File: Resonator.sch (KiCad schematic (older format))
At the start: 29 parts, among them J1 Conn_01x04_Male, SW1 Rotary_Encoder_Switch, SW2 SW_Push, U1 STM32H750VBTx, U2 AT25xxx, U3 IPS240x240, Y1 ABM8G-25.000MHZ-18-D2Y-T

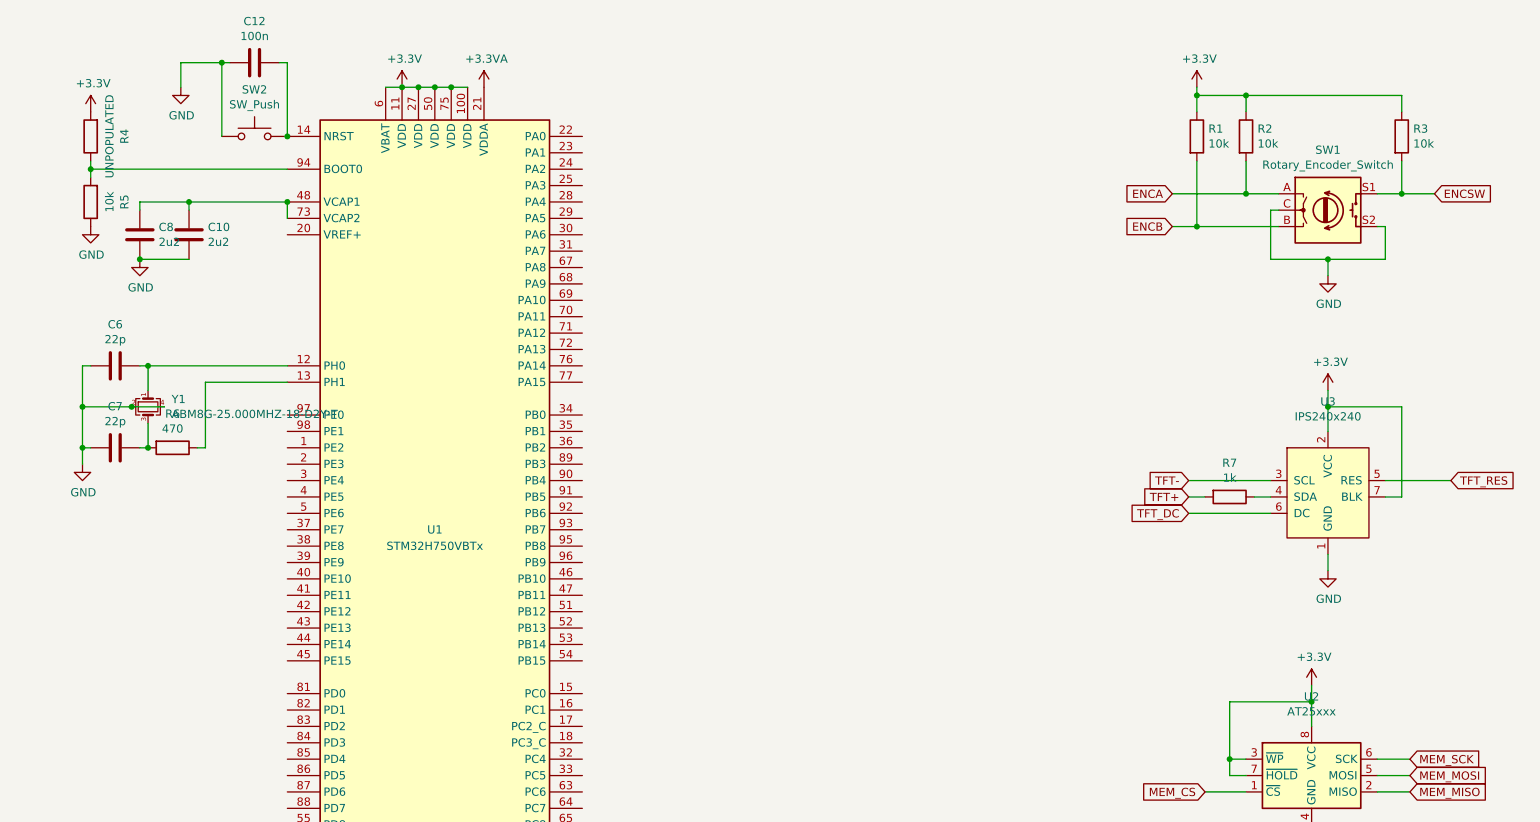
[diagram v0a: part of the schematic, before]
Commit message: Re-annotation.
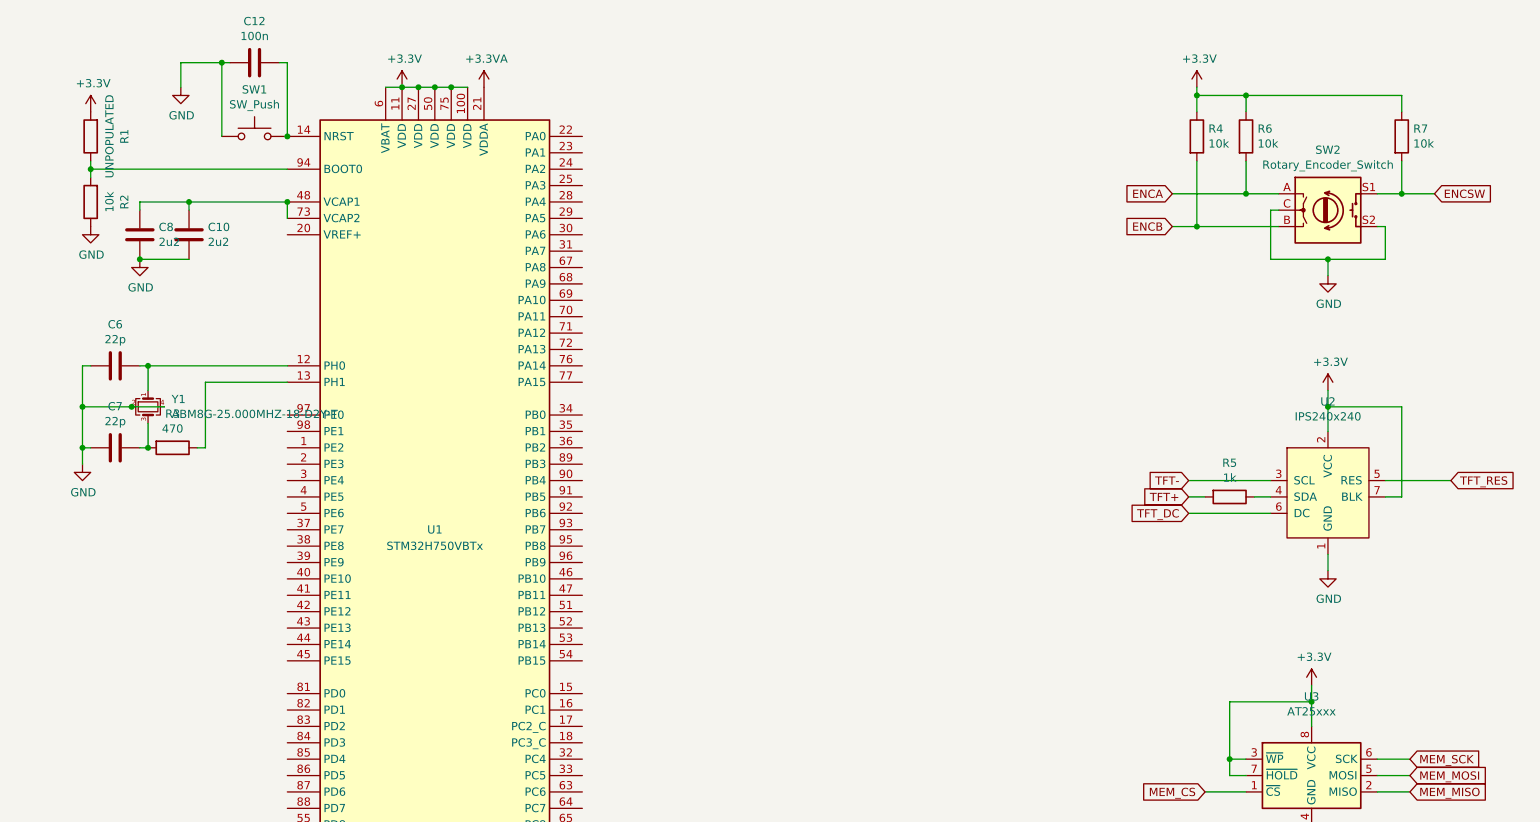
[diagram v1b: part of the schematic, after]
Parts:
- renumbered R4 to R1, R5 to R2, R6 to R3, R1 to R4, R7 to R5, R2 to R6, R3 to R7, SW2 to SW1, SW1 to SW2, U3 to U2, U2 to U3
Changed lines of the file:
@@
 $Descr A3 16535 11693
 encoding utf-8
-Sheet 1 6
+Sheet 1 11
 Title "Resonator"
 Date "2021-11-21"
@@
 Connection ~ 7650 2750
 $Comp
-L power:+3.3V #PWR013
+L power:+3.3V #PWR012
 U 1 1 61D958D9
 P 7650 2750
-F 0 "#PWR013" H 7650 2600 50  0001 C CNN
+F 0 "#PWR012" H 7650 2600 50  0001 C CNN
 F 1 "+3.3V" H 7665 2923 50  0000 C CNN
 F 2 "" H 7650 2750 50  0001 C CNN
@@
 $EndComp
 $Comp
-L power:+3.3VA #PWR016
+L power:+3.3VA #PWR015
 U 1 1 61D96DEA
 P 8150 2750
-F 0 "#PWR016" H 8150 2600 50  0001 C CNN
+F 0 "#PWR015" H 8150 2600 50  0001 C CNN
 F 1 "+3.3VA" H 8165 2923 50  0000 C CNN
 F 2 "" H 8150 2750 50  0001 C CNN
@@
 $EndComp
 $Comp
-L power:GND #PWR012
+L power:GND #PWR011
 U 1 1 61D9B5CB
 P 7550 8250
-F 0 "#PWR012" H 7550 8000 50  0001 C CNN
+F 0 "#PWR011" H 7550 8000 50  0001 C CNN
 F 1 "GND" H 7555 8077 50  0000 C CNN
 F 2 "" H 7550 8250 50  0001 C CNN
@@
 	6950 3550 6950 3450
 $Comp
-L power:GND #PWR010
+L power:GND #PWR09
 U 1 1 61DA19D2
 P 6050 3800
-F 0 "#PWR010" H 6050 3550 50  0001 C CNN
+F 0 "#PWR09" H 6050 3550 50  0001 C CNN
 F 1 "GND" H 6055 3627 50  0000 C CNN
 F 2 "" H 6050 3800 50  0001 C CNN
@@
 Connection ~ 6050 3800
 $Comp
-L power:+3V3 #PWR04
+L power:+3V3 #PWR03
 U 1 1 61DAD533
 P 4050 10300
-F 0 "#PWR04" H 4050 10150 50  0001 C CNN
+F 0 "#PWR03" H 4050 10150 50  0001 C CNN
 F 1 "+3V3" H 4065 10473 50  0000 C CNN
 F 2 "" H 4050 10300 50  0001 C CNN
@@
 	4050 10300 4200 10300
 $Comp
-L power:GND #PWR05
+L power:GND #PWR04
 U 1 1 61DAD53E
 P 4050 10600
-F 0 "#PWR05" H 4050 10350 50  0001 C CNN
+F 0 "#PWR04" H 4050 10350 50  0001 C CNN
 F 1 "GND" H 4055 10427 50  0000 C CNN
 F 2 "" H 4050 10600 50  0001 C CNN
@@
 $EndComp
 $Comp
-L Device:R R4
+L Device:R R1
 U 1 1 61DB7AD0
 P 5750 3050
-F 0 "R4" V 5543 3050 50  0000 C CNN
+F 0 "R1" V 5543 3050 50  0000 C CNN
 F 1 "UNPOPULATED" V 5634 3050 50  0000 C CNN
 F 2 "Resistor_SMD:R_0603_1608Metric" V 5680 3050 50  0001 C CNN
@@
 $EndComp
 $Comp
-L Switch:SW_Push SW2
+L Switch:SW_Push SW1
 U 1 1 61DBD527
 P 6750 3050
-F 0 "SW2" H 6750 3335 50  0000 C CNN
+F 0 "SW1" H 6750 3335 50  0000 C CNN
 F 1 "SW_Push" H 6750 3244 50  0000 C CNN
 F 2 "Button_Switch_THT:SW_PUSH_6mm" H 6750 3250 50  0001 C CNN
@@
 	6950 2600 6900 2600
 $Comp
-L power:GND #PWR011
+L power:GND #PWR010
 U 1 1 61DC8FB1
 P 6300 2750
-F 0 "#PWR011" H 6300 2500 50  0001 C CNN
+F 0 "#PWR010" H 6300 2500 50  0001 C CNN
 F 1 "GND" H 6305 2577 50  0000 C CNN
 F 2 "" H 6300 2750 50  0001 C CNN
@@
 	5700 4700 5700 4450
 $Comp
-L power:GND #PWR07
+L power:GND #PWR06
 U 1 1 61E01E16
 P 5700 5050
-F 0 "#PWR07" H 5700 4800 50  0001 C CNN
+F 0 "#PWR06" H 5700 4800 50  0001 C CNN
 F 1 "GND" H 5705 4877 50  0000 C CNN
 F 2 "" H 5700 5050 50  0001 C CNN
@@
 	7750 10300 7900 10300
 $Comp
-L power:GND #PWR015
+L power:GND #PWR014
 U 1 1 61E8662A
 P 7750 10600
-F 0 "#PWR015" H 7750 10350 50  0001 C CNN
+F 0 "#PWR014" H 7750 10350 50  0001 C CNN
 F 1 "GND" H 7755 10427 50  0000 C CNN
 F 2 "" H 7750 10600 50  0001 C CNN
@@
 	7750 10600 7900 10600
 $Comp
-L power:+3.3VA #PWR014
+L power:+3.3VA #PWR013
 U 1 1 61E8B8BA
 P 7750 10300
-F 0 "#PWR014" H 7750 10150 50  0001 C CNN
+F 0 "#PWR013" H 7750 10150 50  0001 C CNN
 F 1 "+3.3VA" H 7765 10473 50  0000 C CNN
 F 2 "" H 7750 10300 50  0001 C CNN
@@
 	7900 10600 8300 10600
 $Comp
-L Device:R R5
+L Device:R R2
 U 1 1 61ADEFE2
 P 5750 3450
-F 0 "R5" V 5543 3450 50  0000 C CNN
+F 0 "R2" V 5543 3450 50  0000 C CNN
 F 1 "10k" V 5634 3450 50  0000 C CNN
 F 2 "Resistor_SMD:R_0603_1608Metric" V 5680 3450 50  0001 C CNN
@@
 	6100 4800 6100 4950
 $Comp
-L Device:R R6
+L Device:R R3
 U 1 1 61AE0744
 P 6250 4950
-F 0 "R6" V 6043 4950 50  0000 C CNN
+F 0 "R3" V 6043 4950 50  0000 C CNN
 F 1 "470" V 6134 4950 50  0000 C CNN
 F 2 "Resistor_SMD:R_0603_1608Metric" V 6180 4950 50  0001 C CNN
@@
 	5750 3250 5750 3200
 $Comp
-L power:GND #PWR09
+L power:GND #PWR08
 U 1 1 61AF8BC1
 P 5750 3600
-F 0 "#PWR09" H 5750 3350 50  0001 C CNN
+F 0 "#PWR08" H 5750 3350 50  0001 C CNN
 F 1 "GND" H 5755 3427 50  0000 C CNN
 F 2 "" H 5750 3600 50  0001 C CNN
@@
 $EndComp
 $Comp
-L power:+3.3V #PWR08
+L power:+3.3V #PWR07
 U 1 1 61AF9828
 P 5750 2900
-F 0 "#PWR08" H 5750 2750 50  0001 C CNN
+F 0 "#PWR07" H 5750 2750 50  0001 C CNN
 F 1 "+3.3V" H 5765 3073 50  0000 C CNN
 F 2 "" H 5750 2900 50  0001 C CNN
@@
 P 13200 6950
 AR Path="/5DD41DD6/61DD28C6" Ref="U?"  Part="1"
-AR Path="/61DD28C6" Ref="U2"  Part="1"
+AR Path="/61DD28C6" Ref="U3"  Part="1"
 AR Path="/61DB1EC2/61DD28C6" Ref="U?"  Part="1"
-F 0 "U2" H 13200 7431 50  0000 C CNN
+F 0 "U3" H 13200 7431 50  0000 C CNN
 F 1 "AT25xxx" H 13200 7340 50  0000 C CNN
 F 2 "Package_SO:TSSOP-8_4.4x3mm_P0.65mm" H 13200 6950 50  0001 C CNN
@@
 P 13200 7350
 AR Path="/5DD41DD6/61DD28CC" Ref="#PWR?"  Part="1"
-AR Path="/61DD28CC" Ref="#PWR024"  Part="1"
+AR Path="/61DD28CC" Ref="#PWR018"  Part="1"
 AR Path="/61DB1EC2/61DD28CC" Ref="#PWR?"  Part="1"
-F 0 "#PWR024" H 13200 7100 50  0001 C CNN
+F 0 "#PWR018" H 13200 7100 50  0001 C CNN
 F 1 "GND" H 13205 7177 50  0000 C CNN
 F 2 "" H 13200 7350 50  0001 C CNN
@@
 P 13200 6400
 AR Path="/5DD41DD6/61DD28D3" Ref="#PWR?"  Part="1"
-AR Path="/61DD28D3" Ref="#PWR023"  Part="1"
+AR Path="/61DD28D3" Ref="#PWR017"  Part="1"
 AR Path="/61DB1EC2/61DD28D3" Ref="#PWR?"  Part="1"
-F 0 "#PWR023" H 13200 6250 50  0001 C CNN
+F 0 "#PWR017" H 13200 6250 50  0001 C CNN
 F 1 "+3.3V" H 13215 6573 50  0000 C CNN
 F 2 "" H 13200 6400 50  0001 C CNN
@@
 P 13300 3500
 AR Path="/5DD41DD6/61DE3E76" Ref="SW?"  Part="1"
-AR Path="/61DE3E76" Ref="SW1"  Part="1"
+AR Path="/61DE3E76" Ref="SW2"  Part="1"
 AR Path="/61DB1EC2/61DE3E76" Ref="SW?"  Part="1"
-F 0 "SW1" H 13300 3867 50  0000 C CNN
+F 0 "SW2" H 13300 3867 50  0000 C CNN
 F 1 "Rotary_Encoder_Switch" H 13300 3776 50  0000 C CNN
 F 2 "Rotary_Encoder:RotaryEncoder_Alps_EC11E-Switch_Vertical_H20mm" H 13150 3660 50  0001 C CNN
@@
 P 13300 3900
 AR Path="/5DD41DD6/61DE3E7C" Ref="#PWR?"  Part="1"
-AR Path="/61DE3E7C" Ref="#PWR03"  Part="1"
+AR Path="/61DE3E7C" Ref="#PWR019"  Part="1"
 AR Path="/61DB1EC2/61DE3E7C" Ref="#PWR?"  Part="1"
-F 0 "#PWR03" H 13300 3650 50  0001 C CNN
+F 0 "#PWR019" H 13300 3650 50  0001 C CNN
 F 1 "GND" H 13305 3727 50  0000 C CNN
 F 2 "" H 13300 3900 50  0001 C CNN
@@
 P 13750 3050
 AR Path="/61DB1EC2/61DE3E90" Ref="R?"  Part="1"
-AR Path="/61DE3E90" Ref="R3"  Part="1"
-F 0 "R3" H 13820 3096 50  0000 L CNN
+AR Path="/61DE3E90" Ref="R7"  Part="1"
+F 0 "R7" H 13820 3096 50  0000 L CNN
 F 1 "10k" H 13820 3005 50  0000 L CNN
 F 2 "Resistor_SMD:R_0603_1608Metric" V 13680 3050 50  0001 C CNN
@@
 P 12800 3050
 AR Path="/61DB1EC2/61DE3E96" Ref="R?"  Part="1"
-AR Path="/61DE3E96" Ref="R2"  Part="1"
-F 0 "R2" H 12870 3096 50  0000 L CNN
+AR Path="/61DE3E96" Ref="R6"  Part="1"
+F 0 "R6" H 12870 3096 50  0000 L CNN
 F 1 "10k" H 12870 3005 50  0000 L CNN
 F 2 "Resistor_SMD:R_0603_1608Metric" V 12730 3050 50  0001 C CNN
@@
 P 12500 3050
 AR Path="/61DB1EC2/61DE3E9C" Ref="R?"  Part="1"
-AR Path="/61DE3E9C" Ref="R1"  Part="1"
-F 0 "R1" H 12570 3096 50  0000 L CNN
+AR Path="/61DE3E9C" Ref="R4"  Part="1"
+F 0 "R4" H 12570 3096 50  0000 L CNN
 F 1 "10k" H 12570 3005 50  0000 L CNN
 F 2 "Resistor_SMD:R_0603_1608Metric" V 12430 3050 50  0001 C CNN
@@
 P 12500 2750
 AR Path="/61DB1EC2/61DE3EAB" Ref="#PWR?"  Part="1"
-AR Path="/61DE3EAB" Ref="#PWR01"  Part="1"
-F 0 "#PWR01" H 12500 2600 50  0001 C CNN
+AR Path="/61DE3EAB" Ref="#PWR016"  Part="1"
+F 0 "#PWR016" H 12500 2600 50  0001 C CNN
 F 1 "+3.3V" H 12515 2923 50  0000 C CNN
 F 2 "" H 12500 2750 50  0001 C CNN
@@
 P 5550 9350
 AR Path="/5DD41DD6/61DED307" Ref="#PWR?"  Part="1"
-AR Path="/61DED307" Ref="#PWR06"  Part="1"
+AR Path="/61DED307" Ref="#PWR05"  Part="1"
 AR Path="/61DB1EC2/61DED307" Ref="#PWR?"  Part="1"
-F 0 "#PWR06" H 5550 9100 50  0001 C CNN
+F 0 "#PWR05" H 5550 9100 50  0001 C CNN
 F 1 "GND" H 5555 9177 50  0000 C CNN
 F 2 "" H 5550 9350 50  0001 C CNN
@@
 P 12700 5250
 AR Path="/5DD41DD6/61E13169" Ref="R?"  Part="1"
-AR Path="/61E13169" Ref="R7"  Part="1"
+AR Path="/61E13169" Ref="R5"  Part="1"
 AR Path="/61DB1EC2/61E13169" Ref="R?"  Part="1"
-F 0 "R7" V 12493 5250 50  0000 C CNN
+F 0 "R5" V 12493 5250 50  0000 C CNN
 F 1 "1k" V 12584 5250 50  0000 C CNN
 F 2 "Resistor_SMD:R_0603_1608Metric" V 12630 5250 50  0001 C CNN
@@
 P 13300 5700
 AR Path="/5DD41DD6/61E13170" Ref="#PWR?"  Part="1"
-AR Path="/61E13170" Ref="#PWR026"  Part="1"
+AR Path="/61E13170" Ref="#PWR021"  Part="1"
 AR Path="/61DB1EC2/61E13170" Ref="#PWR?"  Part="1"
-F 0 "#PWR026" H 13300 5450 50  0001 C CNN
+F 0 "#PWR021" H 13300 5450 50  0001 C CNN
 F 1 "GND" H 13305 5527 50  0000 C CNN
 F 2 "" H 13300 5700 50  0001 C CNN
@@
 P 13300 4600
 AR Path="/5DD41DD6/61E13177" Ref="#PWR?"  Part="1"
-AR Path="/61E13177" Ref="#PWR025"  Part="1"
+AR Path="/61E13177" Ref="#PWR020"  Part="1"
 AR Path="/61DB1EC2/61E13177" Ref="#PWR?"  Part="1"
-F 0 "#PWR025" H 13300 4450 50  0001 C CNN
+F 0 "#PWR020" H 13300 4450 50  0001 C CNN
 F 1 "+3.3V" H 13315 4773 50  0000 C CNN
 F 2 "" H 13300 4600 50  0001 C CNN
@@
 TFT_RES
 $Comp
-L IPS240x240:IPS240x240 U3
+L IPS240x240:IPS240x240 U2
 U 1 1 61E39E11
 P 13150 4400
-F 0 "U3" H 13300 4131 50  0000 C CNN
+F 0 "U2" H 13300 4131 50  0000 C CNN
 F 1 "IPS240x240" H 13300 4040 50  0000 C CNN
 F 2 "" H 13150 4400 50  0001 C CNN
@@
 	2550 5950 2650 5950
 $Comp
-L power:GND #PWR02
+L power:GND #PWR01
 U 1 1 61E78173
 P 1750 6000
-F 0 "#PWR02" H 1750 5750 50  0001 C CNN
+F 0 "#PWR01" H 1750 5750 50  0001 C CNN
 F 1 "GND" H 1755 5827 50  0000 C CNN
 F 2 "" H 1750 6000 50  0001 C CNN
@@
 	2550 6400 2650 6400
 $Comp
-L power:GND #PWR?
+L power:GND #PWR02
 U 1 1 621F67D5
 P 1750 6450
-F 0 "#PWR?" H 1750 6200 50  0001 C CNN
+F 0 "#PWR02" H 1750 6200 50  0001 C CNN
 F 1 "GND" H 1755 6277 50  0000 C CNN
 F 2 "" H 1750 6450 50  0001 C CNN
